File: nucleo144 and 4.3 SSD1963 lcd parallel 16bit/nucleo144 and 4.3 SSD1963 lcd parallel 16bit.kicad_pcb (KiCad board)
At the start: 2 copper layers, 100 x 70 mm, 9 parts, among them U1 NUCLEO144, U2 AMS1117-3.3

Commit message: Signed-off-by: DamianPodrazaCode <damian.podraza@gmail.com>
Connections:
- U1 pad 2: SD__MISO -> SD_MISO
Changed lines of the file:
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@@
   (net 136 "unconnected-(TFT1-NC-Pad36)")
   (net 137 "3.3V")
-  (net 138 "SD__MISO")
   (footprint "zombie_nucleo:ST_Morpho_Connector_144_Short" (layer "F.Cu")
     (at 204.4 63.24 -90)
@@
       (net 133 "SD_CLK") (pinfunction "PC10") (pintype "bidirectional"))
     (pad "2" thru_hole circle (at 2.54 0 270) (size 1.7 1.7) (drill 1) (layers "*.Cu" "*.Mask")
-      (net 138 "SD__MISO") (pinfunction "PC11") (pintype "bidirectional"))
+      (net 134 "SD_MISO") (pinfunction "PC11") (pintype "bidirectional"))
     (pad "3" thru_hole circle (at 0 2.54 270) (size 1.7 1.7) (drill 1) (layers "*.Cu" "*.Mask")
       (net 132 "SD_MOSI") (pinfunction "PC12") (pintype "bidirectional"))

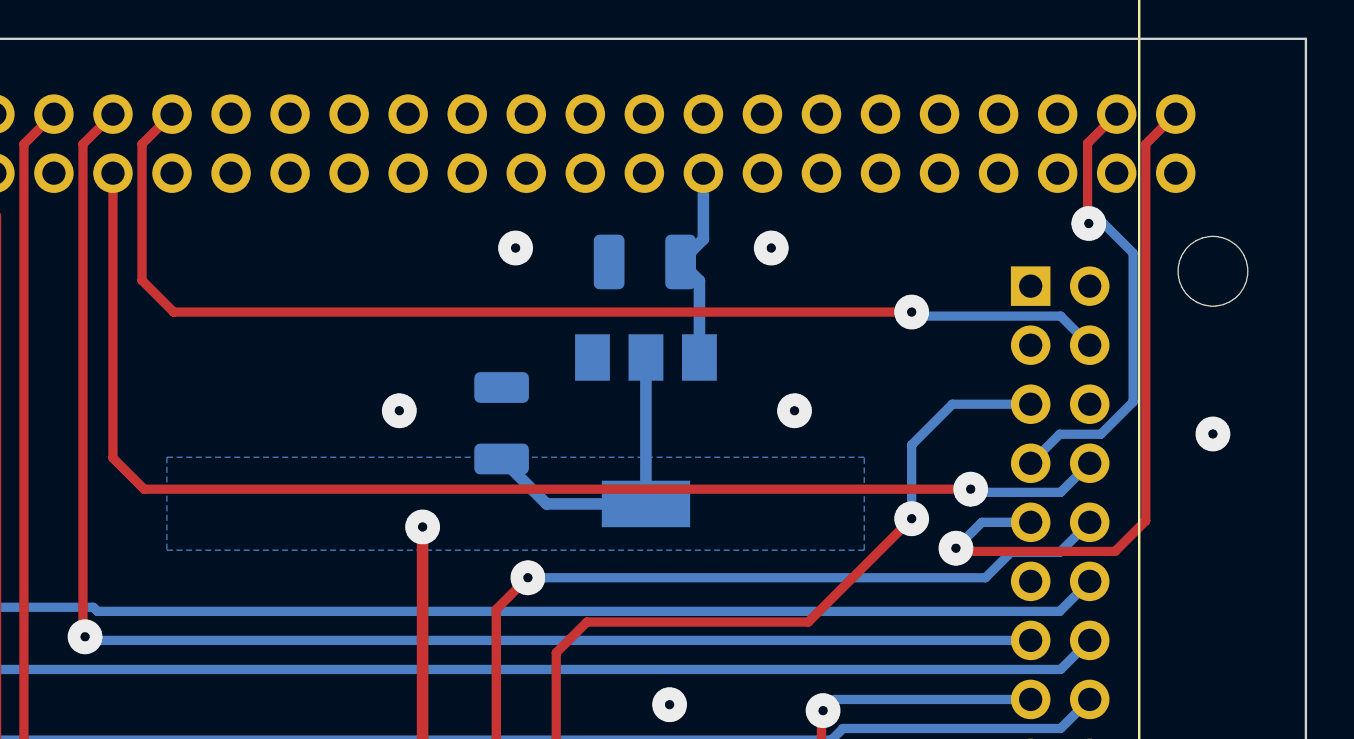
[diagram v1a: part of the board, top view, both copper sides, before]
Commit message: Signed-off-by: DamianPodrazaCode <damian.podraza@gmail.com>
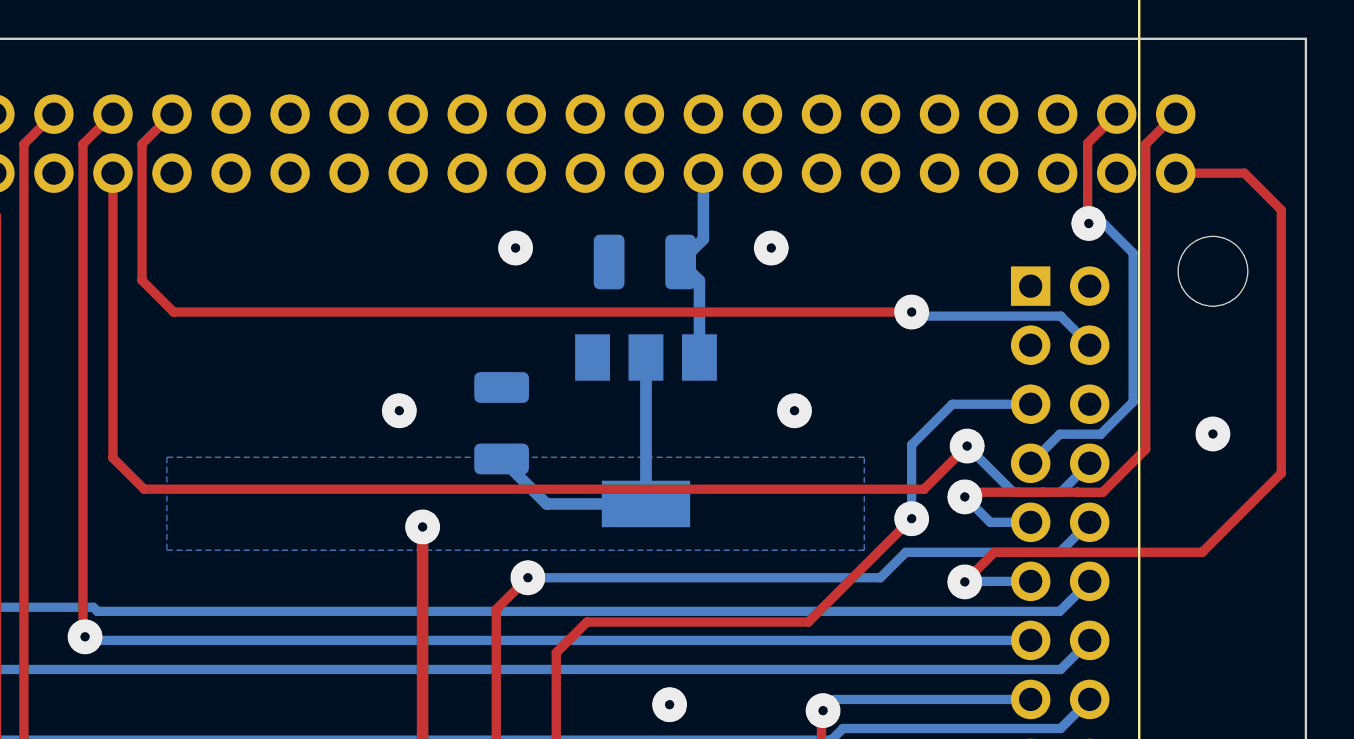
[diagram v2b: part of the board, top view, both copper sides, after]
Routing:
- net SD_MISO: track 0.00 -> 34.9 mm, vias 0 -> 1
- net SD_CLK: track 30.5 -> 26.9 mm
- net LCD_RST: track 55.4 -> 56.9 mm
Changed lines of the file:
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@@
   (segment (start 199.41 84.63) (end 158.011346 84.63) (width 0.4) (layer "B.Cu") (net 38))
   (segment (start 157.836346 84.455) (end 147.32 84.455) (width 0.4) (layer "B.Cu") (net 38))
-  (segment (start 195.58 79.375) (end 160.02 79.375) (width 0.4) (layer "F.Cu") (net 50))
   (segment (start 158.68 78.035) (end 158.68 65.78) (width 0.4) (layer "F.Cu") (net 50))
+  (segment (start 195.4276 77.5208) (end 193.5734 79.375) (width 0.4) (layer "F.Cu") (net 50))
+  (segment (start 193.5734 79.375) (end 160.02 79.375) (width 0.4) (layer "F.Cu") (net 50))
   (segment (start 160.02 79.375) (end 158.68 78.035) (width 0.4) (layer "F.Cu") (net 50))
-  (via (at 195.58 79.375) (size 1.5) (drill 0.4) (layers "F.Cu" "B.Cu") (net 50))
-  (segment (start 195.715 79.51) (end 195.58 79.375) (width 0.4) (layer "B.Cu") (net 50))
-  (segment (start 200.7 78.26) (end 199.45 79.51) (width 0.4) (layer "B.Cu") (net 50))
-  (segment (start 199.45 79.51) (end 195.715 79.51) (width 0.4) (layer "B.Cu") (net 50))
+  (via (at 195.4276 77.5208) (size 1.5) (drill 0.4) (layers "F.Cu" "B.Cu") (net 50))
+  (segment (start 197.4168 79.51) (end 199.45 79.51) (width 0.4) (layer "B.Cu") (net 50))
+  (segment (start 195.4276 77.5208) (end 197.4168 79.51) (width 0.4) (layer "B.Cu") (net 50))
+  (segment (start 199.45 79.51) (end 200.7 78.26) (width 0.4) (layer "B.Cu") (net 50))
   (segment (start 150.15 112.8205) (end 150.15 120.85) (width 0.4) (layer "F.Cu") (net 91))
   (segment (start 150.15 120.85) (end 148.52 122.48) (width 0.4) (layer "F.Cu") (net 91))
@@
   (segment (start 175.17 84.545) (end 175.17 125.45) (width 0.4) (layer "F.Cu") (net 109))
   (via (at 176.53 83.185) (size 1.5) (drill 0.4) (layers "F.Cu" "B.Cu") (net 109))
-  (segment (start 176.53 83.185) (end 196.215 83.185) (width 0.4) (layer "B.Cu") (net 109))
-  (segment (start 196.215 83.185) (end 197.31 82.09) (width 0.4) (layer "B.Cu") (net 109))
+  (segment (start 192.7888 82.09) (end 199.41 82.09) (width 0.4) (layer "B.Cu") (net 109))
   (segment (start 199.41 82.09) (end 200.7 80.8) (width 0.4) (layer "B.Cu") (net 109))
-  (segment (start 197.31 82.09) (end 199.41 82.09) (width 0.4) (layer "B.Cu") (net 109))
+  (segment (start 191.6938 83.185) (end 192.7888 82.09) (width 0.4) (layer "B.Cu") (net 109))
+  (segment (start 176.53 83.185) (end 191.6938 83.185) (width 0.4) (layer "B.Cu") (net 109))
   (segment (start 158.68 120.32) (end 158.68 124.2) (width 0.4) (layer "F.Cu") (net 110))
   (segment (start 159 120) (end 158.68 120.32) (width 0.4) (layer "F.Cu") (net 110))
@@
   (segment (start 202.565 69.215) (end 201.295 67.945) (width 0.4) (layer "B.Cu") (net 132))
   (segment (start 201.177767 77.01) (end 202.565 75.622767) (width 0.4) (layer "B.Cu") (net 132))
-  (segment (start 201.795 82.05) (end 203.11 80.735) (width 0.4) (layer "F.Cu") (net 133))
-  (segment (start 195.08 82.05) (end 201.795 82.05) (width 0.4) (layer "F.Cu") (net 133))
+  (segment (start 195.326 79.7052) (end 195.5292 79.502) (width 0.4) (layer "F.Cu") (net 133))
   (segment (start 203.11 64.53) (end 204.4 63.24) (width 0.4) (layer "F.Cu") (net 133))
-  (segment (start 194.945 81.915) (end 195.08 82.05) (width 0.4) (layer "F.Cu") (net 133))
-  (segment (start 203.11 80.735) (end 203.11 64.53) (width 0.4) (layer "F.Cu") (net 133))
-  (via (at 194.945 81.915) (size 1.5) (drill 0.4) (layers "F.Cu" "B.Cu") (net 133))
-  (segment (start 198.16 80.8) (end 196.06 80.8) (width 0.4) (layer "B.Cu") (net 133))
-  (segment (start 196.06 80.8) (end 194.945 81.915) (width 0.4) (layer "B.Cu") (net 133))
+  (segment (start 197.642233 79.51) (end 198.677767 79.51) (width 0.4) (layer "F.Cu") (net 133))
+  (segment (start 198.685767 79.502) (end 200.174233 79.502) (width 0.4) (layer "F.Cu") (net 133))
+  (segment (start 203.11 77.657767) (end 203.11 64.53) (width 0.4) (layer "F.Cu") (net 133))
+  (segment (start 201.257767 79.51) (end 203.11 77.657767) (width 0.4) (layer "F.Cu") (net 133))
+  (segment (start 200.182233 79.51) (end 201.257767 79.51) (width 0.4) (layer "F.Cu") (net 133))
+  (segment (start 195.5292 79.502) (end 197.634233 79.502) (width 0.4) (layer "F.Cu") (net 133))
+  (segment (start 198.677767 79.51) (end 198.685767 79.502) (width 0.4) (layer "F.Cu") (net 133))
+  (segment (start 197.634233 79.502) (end 197.642233 79.51) (width 0.4) (layer "F.Cu") (net 133))
+  (segment (start 200.174233 79.502) (end 200.182233 79.51) (width 0.4) (layer "F.Cu") (net 133))
+  (via (at 195.326 79.7052) (size 1.5) (drill 0.4) (layers "F.Cu" "B.Cu") (net 133))
+  (segment (start 195.326 79.7052) (end 196.4208 80.8) (width 0.4) (layer "B.Cu") (net 133))
+  (segment (start 196.4208 80.8) (end 198.16 80.8) (width 0.4) (layer "B.Cu") (net 133))
+  (segment (start 208.9404 67.3608) (end 207.3596 65.78) (width 0.4) (layer "F.Cu") (net 134))
+  (segment (start 208.9404 78.6892) (end 208.9404 67.3608) (width 0.4) (layer "F.Cu") (net 134))
+  (segment (start 195.326 83.3628) (end 196.5988 82.09) (width 0.4) (layer "F.Cu") (net 134))
+  (segment (start 207.3596 65.78) (end 204.4 65.78) (width 0.4) (layer "F.Cu") (net 134))
+  (segment (start 205.5396 82.09) (end 208.9404 78.6892) (width 0.4) (layer "F.Cu") (net 134))
+  (segment (start 196.5988 82.09) (end 205.5396 82.09) (width 0.4) (layer "F.Cu") (net 134))
+  (via (at 195.326 83.3628) (size 1.5) (drill 0.4) (layers "F.Cu" "B.Cu") (net 134))
+  (segment (start 198.16 83.34) (end 195.3488 83.34) (width 0.4) (layer "B.Cu") (net 134))
+  (segment (start 195.3488 83.34) (end 195.326 83.3628) (width 0.4) (layer "B.Cu") (net 134))
   (segment (start 172 121) (end 172 81) (width 0.5) (layer "F.Cu") (net 137))
   (via (at 172 121) (size 1.5) (drill 0.4) (layers "F.Cu" "B.Cu") (net 137))
